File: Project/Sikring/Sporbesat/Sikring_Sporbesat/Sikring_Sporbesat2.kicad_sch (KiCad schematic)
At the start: 16 parts, among them J1 Screw_Terminal_01x02, J2 Screw_Terminal_01x02, J3 Conn_01x05_Socket, Q1 BC857, U1 PC847

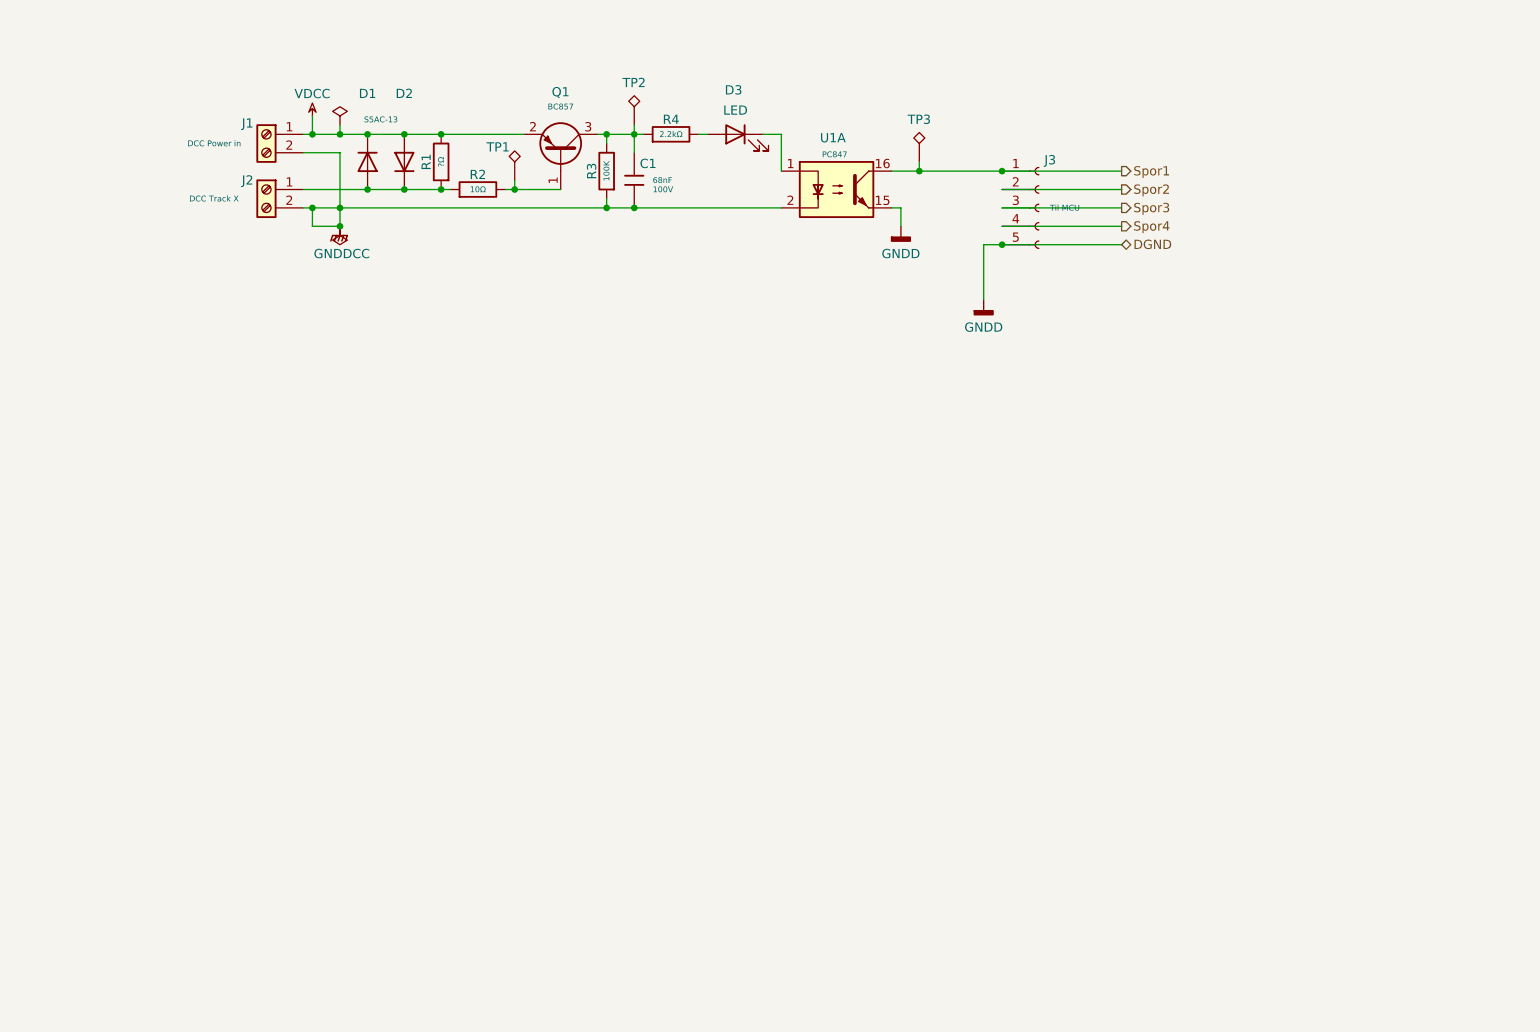
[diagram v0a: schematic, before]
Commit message: Sikringsanlæg - Sporbesat
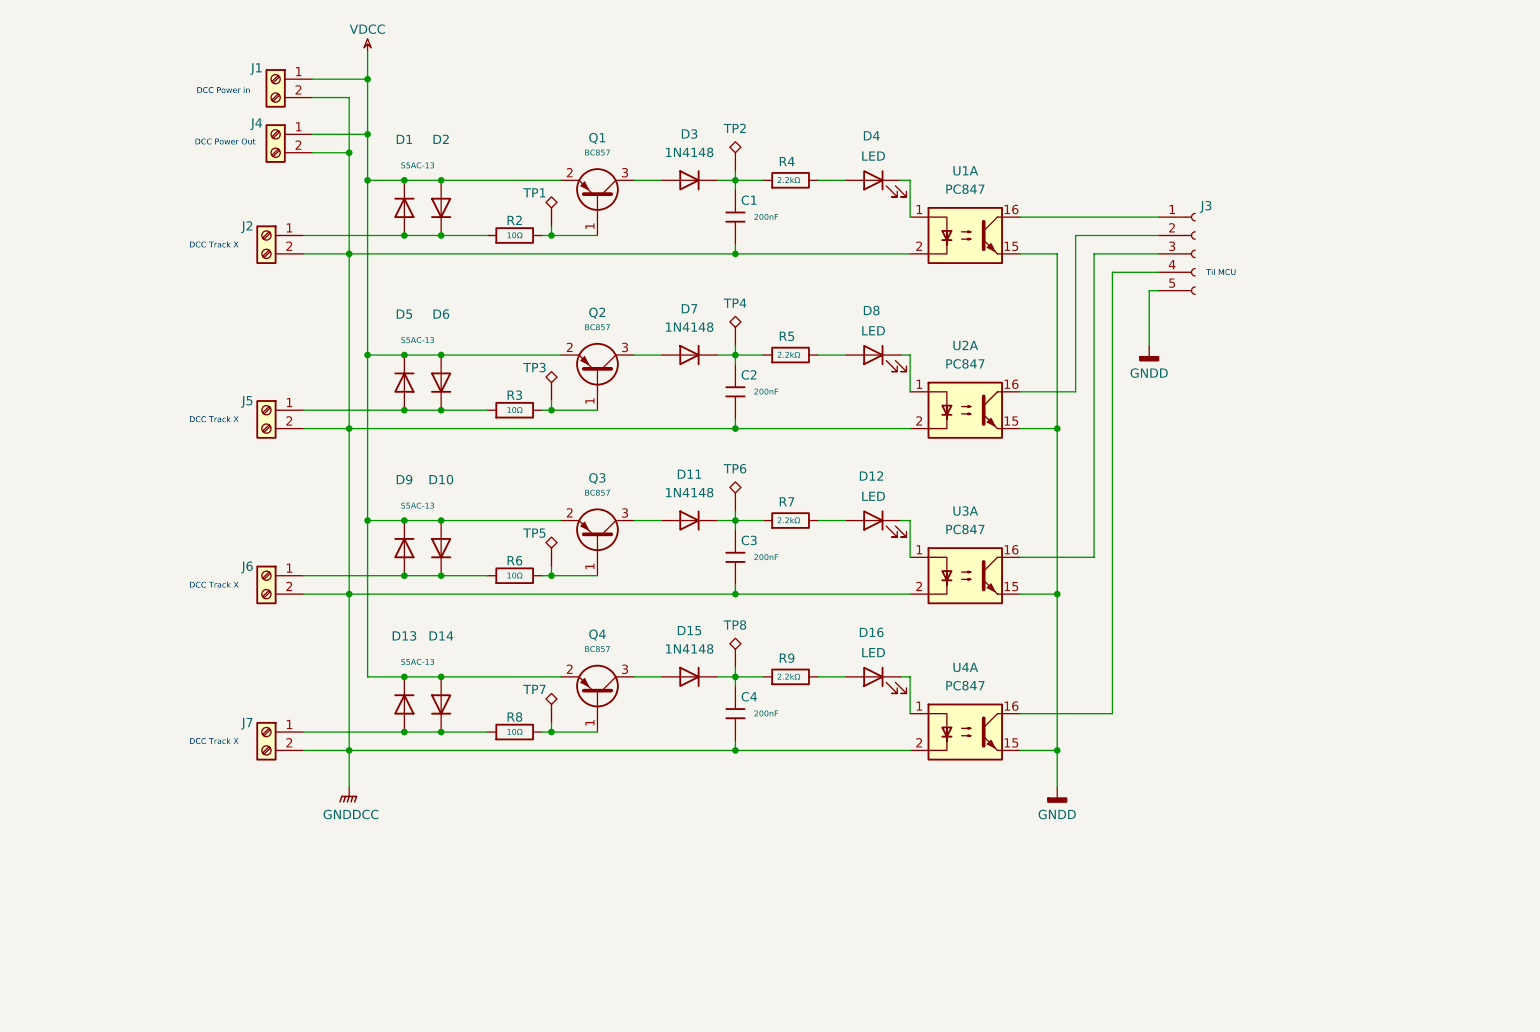
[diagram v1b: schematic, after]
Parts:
- removed R1: ?Ω, PCM_JLCPCB:R_0805, symbol PCM_JLCPCB-Resistors:0805,1.8kΩ
- added C2, C3, C4: 200nF, PCM_JLCPCB:C_0805, symbol PCM_JLCPCB-Capacitors:0805,470nF
- added D10, D13, D14, D5, D6, D9: S5AC-13, Diode_SMD:D_MELF_Handsoldering, symbol Device:D
- added D11, D15, D3, D7: 1N4148, Diode_THT:D_DO-35_SOD27_P7.62mm_Horizontal, symbol Diode:1N4148
- added D12, D16, D8: LED, LED_SMD:LED_0805_2012Metric, symbol Device:LED
- added J4: Screw_Terminal_01x02, Package_SON:WSON-8-1EP_6x5mm_P1.27mm_EP3.4x4mm, symbol Connector:Screw_Terminal_01x02
- added J5, J6, J7: Screw_Terminal_01x02, symbol Connector:Screw_Terminal_01x02
- added Q2, Q3, Q4: BC857, Package_TO_SOT_SMD:SOT-23, symbol Transistor_BJT:BC857
- added R5, R7, R9: 2.2kΩ, PCM_JLCPCB:R_0805, symbol PCM_JLCPCB-Resistors:0805,1.8kΩ
- added R6, R8: 10Ω, PCM_JLCPCB:R_0805, symbol PCM_JLCPCB-Resistors:0805,1.8kΩ
- added TP4, TP6, TP8: U1A_Collector, TestPoint:TestPoint_Loop_D2.60mm_Drill1.4mm_Beaded, symbol Connector:TestPoint_Alt
- added TP5, TP7: Q1_Basic, TestPoint:TestPoint_Loop_D2.60mm_Drill1.4mm_Beaded, symbol Connector:TestPoint_Alt
- added U2, U3, U4: PC847, Package_DIP:DIP-16_W7.62mm, symbol Isolator:PC847
- C1: value 68nF -> 200nF
- R3: value 100K -> 10Ω
- TP2: value Q1_Collector -> U1A_Collector
- TP3: value U1A_Collector -> Q1_Basic
- renumbered D3 to D4
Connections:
- net GNDD: now also U2.15, U3.15, U4.15
- net GNDDCC: now also C2.2, C3.2, C4.2, J4.2 (Pin_2), J5.2 (Pin_2), J6.2 (Pin_2), J7.2 (Pin_2), U2.2, U3.2, U4.2; no longer R3.1
- net VDCC: now also D10.2 (A), D13.1 (K), D14.2 (A), D5.1 (K), D6.2 (A), D9.1 (K), J4.1 (Pin_1), Q2.2 (E), Q3.2 (E), Q4.2 (E)
- net at C1.1, R4.1, TP2.1: now also D3.1 (K); no longer Q1.3 (C), R3.2
- net Spor1: no longer names the net of J3.1 (Pin_1), U1.16
- net Spor1: no longer TP3.1
- net Spor2: no longer names the net of J3.2 (Pin_2)
- net Spor2: now also U2.16
- net Spor3: no longer names the net of J3.3 (Pin_3)
- net Spor3: now also U3.16
- net Spor4: no longer names the net of J3.4 (Pin_4)
- net Spor4: now also U4.16
- new net: D12.1 (K), U3.1
- new net: C2.1, D7.1 (K), R5.1, TP4.1
- new net: D7.2 (A), Q2.3 (C)
- new net: D5.2 (A), D6.1 (K), J5.1 (Pin_1), R3.1
- new net: Q4.1 (B), R8.2, TP7.1
- new net: D10.1 (K), D9.2 (A), J6.1 (Pin_1), R6.1
- new net: D13.2 (A), D14.1 (K), J7.1 (Pin_1), R8.1
- new net: C4.1, D15.1 (K), R9.1, TP8.1
- new net: D3.2 (A), Q1.3 (C)
- new net: Q2.1 (B), R3.2, TP3.1
- new net: C3.1, D11.1 (K), R7.1, TP6.1
- new net: D11.2 (A), Q3.3 (C)
- new net: D16.1 (K), U4.1
- new net: Q3.1 (B), R6.2, TP5.1
- new net: D15.2 (A), Q4.3 (C)
- new net: D16.2 (A), R9.2
- new net: D12.2 (A), R7.2
- new net: D8.2 (A), R5.2
- new net: D8.1 (K), U2.1
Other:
- note added: "DCC Power Out"
- moved on the sheet: C1, D1, D2, D4, J1, J2, J3, Q1, R2, R4, TP1

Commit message: canbus
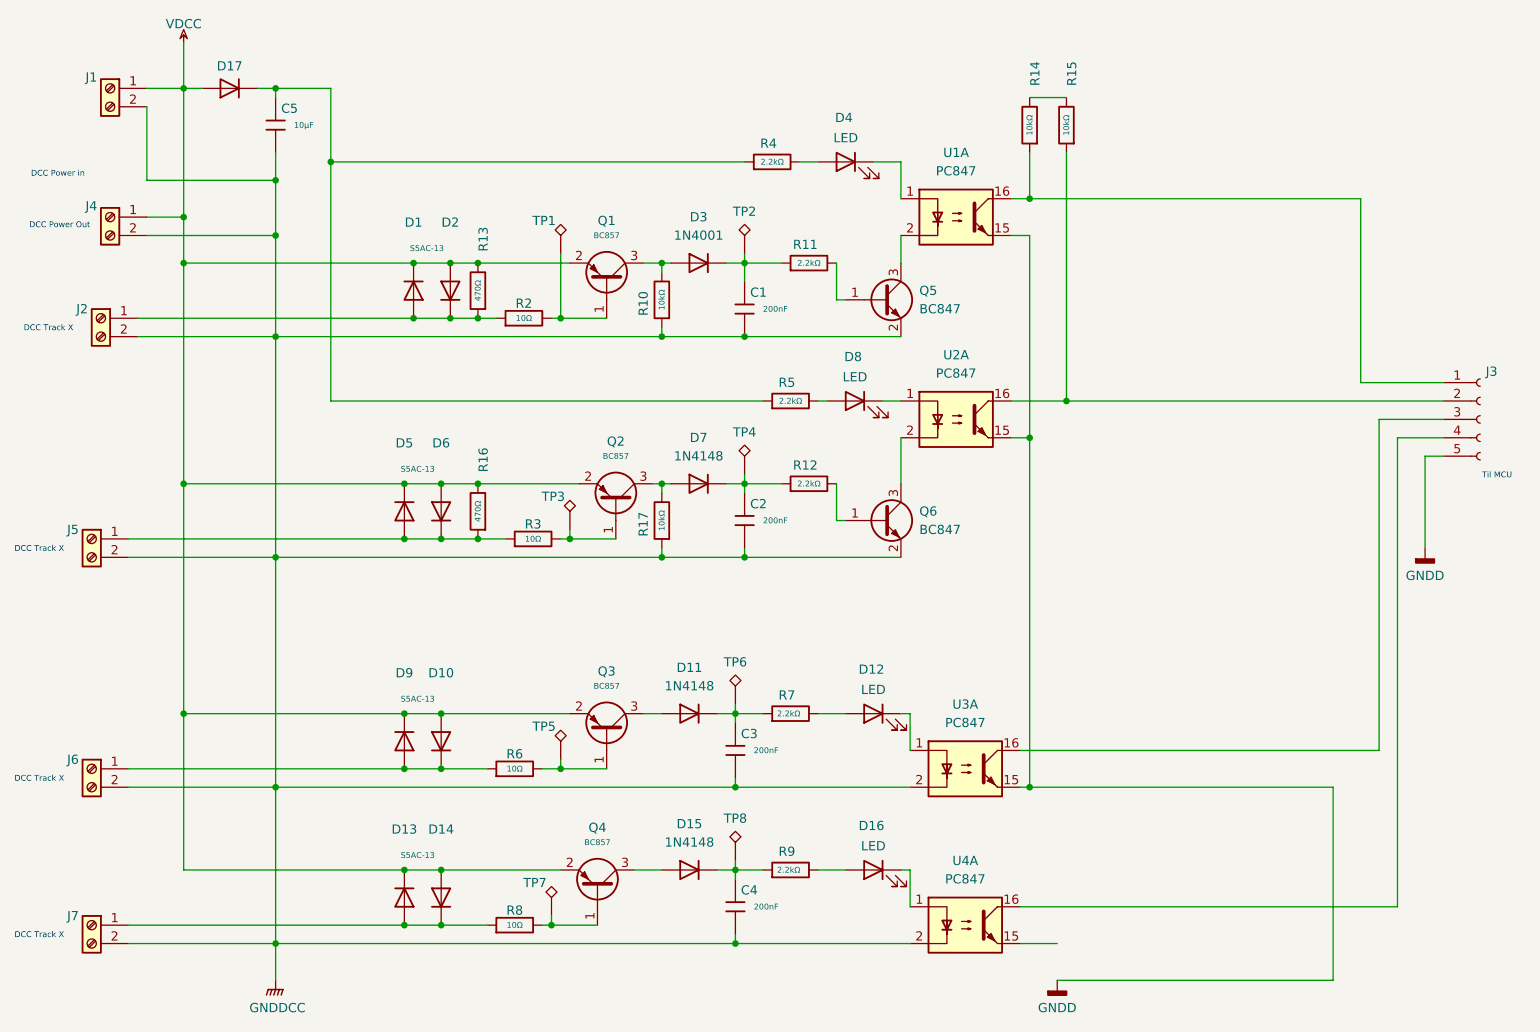
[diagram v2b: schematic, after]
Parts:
- added C5: 10µF, PCM_JLCPCB:C_0805, symbol PCM_JLCPCB-Capacitors:0805,470nF
- added D17: S5AC-13, Diode_SMD:D_MELF_Handsoldering, symbol Device:D
- added Q5, Q6: BC847, Package_TO_SOT_SMD:SOT-23, symbol Transistor_BJT:BC847
- added R10, R14, R15, R17: 10kΩ, PCM_JLCPCB:R_0805, symbol PCM_JLCPCB-Resistors:0805,1.8kΩ
- added R11, R12: 2.2kΩ, PCM_JLCPCB:R_0805, symbol PCM_JLCPCB-Resistors:0805,1.8kΩ
- added R13, R16: 470Ω, PCM_JLCPCB:R_0805, symbol PCM_JLCPCB-Resistors:0805,1.8kΩ
- D3: value 1N4148 -> 1N4001
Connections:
- net GNDD: no longer U4.15
- net GNDDCC: now also C5.2, Q5.2 (E), Q6.2 (E), R10.1, R17.1; no longer U1.2, U2.2
- net VDCC: now also D17.2 (A), R13.2, R16.2
- net at C2.1, D7.1 (K), TP4.1: now also R12.1; no longer R5.1
- net at D7.2 (A), Q2.3 (C): now also R17.2
- net at D5.2 (A), D6.1 (K), J5.1 (Pin_1)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: now also R16.1
- net at D3.2 (A), Q1.3 (C): now also R10.2
- net at J3.1 (Pin_1), U1.16: now also R14.1
- net at C1.1, D3.1 (K), TP2.1: now also R11.1; no longer R4.1
- net at D1.2 (A), D2.1 (K), J2.1 (Pin_1)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: now also R13.1
- net at J3.2 (Pin_2), U2.16: now also R15.1
- new net: C5.1, D17.1 (K), R4.1, R5.1
- new net: Q6.1 (B), R12.2
- new net: Q6.3 (C), U2.2
- new net: R14.2, R15.2
- new net: Q5.3 (C), U1.2
- new net: Q5.1 (B), R11.2
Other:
- moved on the sheet: C1, C2, C3, C4, D1, D10, D11, D12, D13, D14, D15, D16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

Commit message: Beskrivelse af functionen af Sporbesat detektor
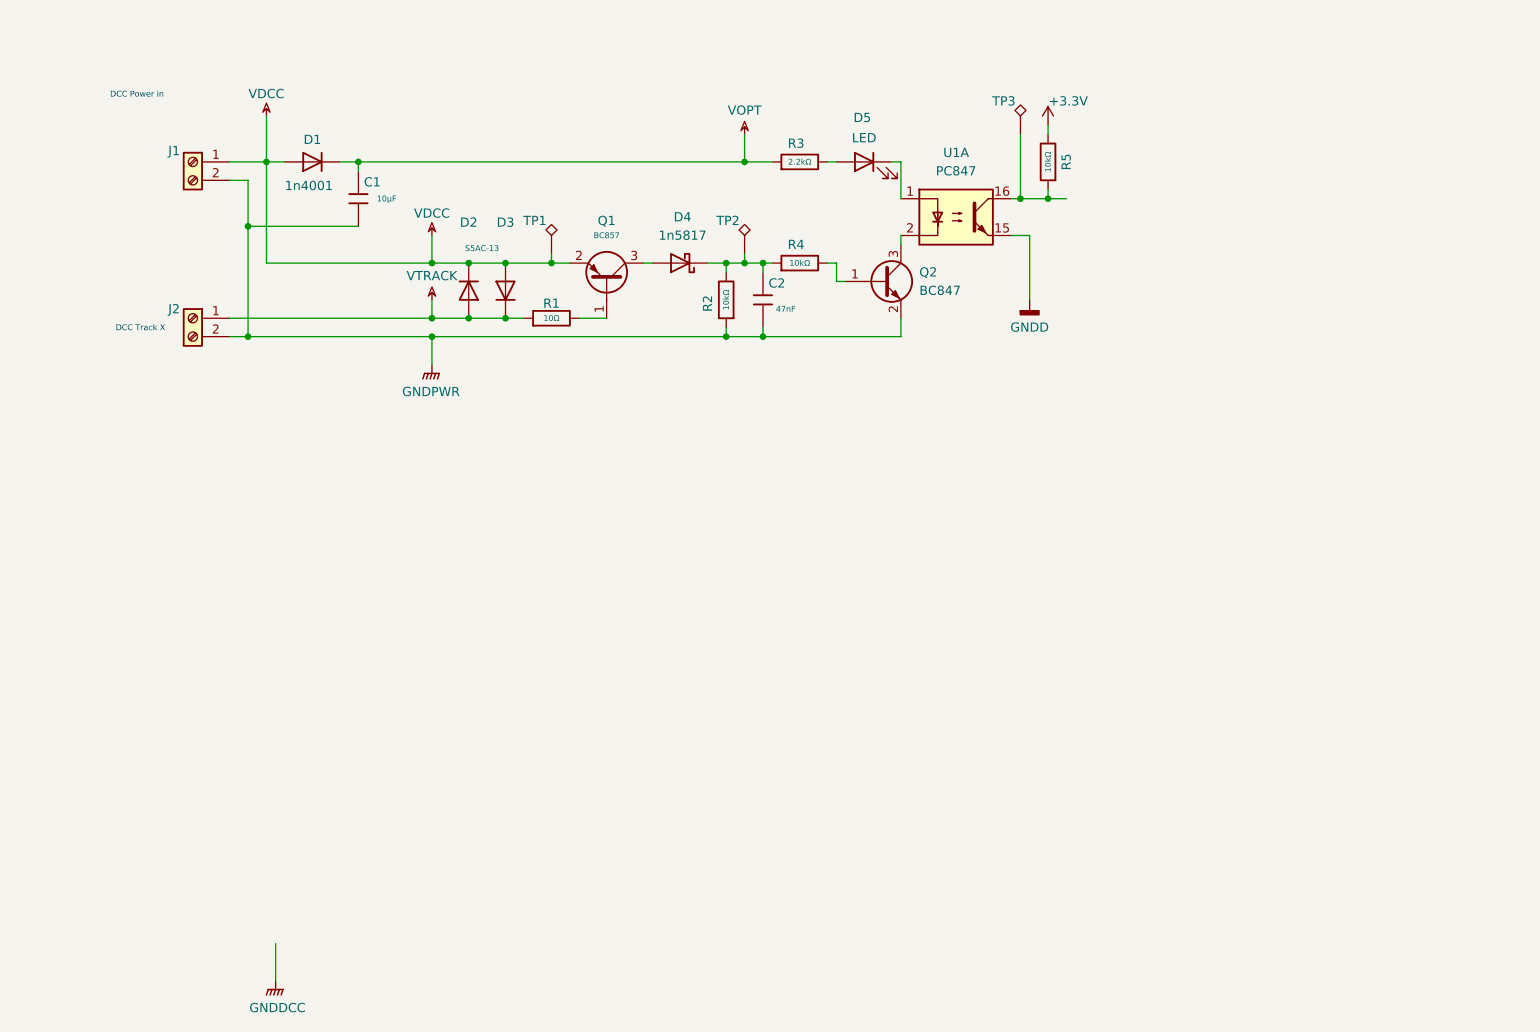
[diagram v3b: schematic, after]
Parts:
- removed C2, C3, C4: 200nF, PCM_JLCPCB:C_0805, symbol PCM_JLCPCB-Capacitors:0805,470nF
- removed D10, D13, D14, D5, D6, D9: S5AC-13, Diode_SMD:D_MELF_Handsoldering, symbol Device:D
- removed D11, D15, D7: 1N4148, Diode_THT:D_DO-35_SOD27_P7.62mm_Horizontal, symbol Diode:1N4148
- removed D12, D16, D8: LED, LED_SMD:LED_0805_2012Metric, symbol Device:LED
- removed D3: 1N4001, Diode_THT:D_DO-35_SOD27_P7.62mm_Horizontal, symbol Diode:1N4148
- removed J3: Conn_01x05_Socket, symbol Connector:Conn_01x05_Socket
- removed J4: Screw_Terminal_01x02, Package_SON:WSON-8-1EP_6x5mm_P1.27mm_EP3.4x4mm, symbol Connector:Screw_Terminal_01x02
- removed J5, J6, J7: Screw_Terminal_01x02, symbol Connector:Screw_Terminal_01x02
- removed Q2, Q3, Q4: BC857, Package_TO_SOT_SMD:SOT-23, symbol Transistor_BJT:BC857
- removed Q6: BC847, Package_TO_SOT_SMD:SOT-23, symbol Transistor_BJT:BC847
- removed R12, R5, R7, R9: 2.2kΩ, PCM_JLCPCB:R_0805, symbol PCM_JLCPCB-Resistors:0805,1.8kΩ
- removed R13, R16: 470Ω, PCM_JLCPCB:R_0805, symbol PCM_JLCPCB-Resistors:0805,1.8kΩ
- removed R15, R17: 10kΩ, PCM_JLCPCB:R_0805, symbol PCM_JLCPCB-Resistors:0805,1.8kΩ
- removed R3, R6, R8: 10Ω, PCM_JLCPCB:R_0805, symbol PCM_JLCPCB-Resistors:0805,1.8kΩ
- removed TP2, TP4, TP6, TP8: U1A_Collector, TestPoint:TestPoint_Loop_D2.60mm_Drill1.4mm_Beaded, symbol Connector:TestPoint_Alt
- removed TP5, TP7: Q1_Basic, TestPoint:TestPoint_Loop_D2.60mm_Drill1.4mm_Beaded, symbol Connector:TestPoint_Alt
- removed U2, U3, U4: PC847, Package_DIP:DIP-16_W7.62mm, symbol Isolator:PC847
- added D4: 1n5817, symbol Device:D_Schottky
- added TP1: Q1_Basic, TestPoint:TestPoint_Loop_D2.60mm_Drill1.4mm_Beaded, symbol Connector:TestPoint_Alt
- C2: renamed from C1; value 200nF -> 47nF
- D1: renamed from D17; value S5AC-13 -> 1n4001
- R4: renamed from R11; value 2.2kΩ -> 10kΩ
- renumbered C5 to C1, D1 to D2, D2 to D3, D4 to D5, Q5 to Q2, R2 to R1, R10 to R2, R4 to R3, R14 to R5, TP1 to TP2
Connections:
- net GNDDCC: no longer C1.2, C2.2, J1.2 (Pin_2), J2.2 (Pin_2), Q2.2 (E), R2.1
- net VDCC: now also TP1.1
- net VOPT: now reaches C1.1, D1.1 (K), R3.1
- net +3.3V: now reaches R5.2
- net at Q1.1 (B), R1.2: no longer TP2.1
- net at Q1.3 (C): now also D4.2 (A); no longer R2.2
- net at R5.1, U1.16: now also TP3.1
- net at C2.1, R4.1: now also R2.2, TP2.1, D4.1 (K)
- net VTRACK: now reaches D2.2 (A), D3.1 (K), J2.1 (Pin_1), R1.1
- new net GNDPWR: C1.2, C2.2, J1.2 (Pin_2), J2.2 (Pin_2), Q2.2 (E), R2.1
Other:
- note removed: "DCC Power Out"
- note removed: "Til MCU"
- moved on the sheet: C1, C2, D1, D2, D3, D5, J1, J2, Q2, R1, R2, R3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
